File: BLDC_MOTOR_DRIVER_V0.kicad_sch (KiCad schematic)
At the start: 47 parts, among them J1 Conn_01x05_Pin, J10 Conn_01x01_Socket, J2 Conn_01x01_Socket, J3 Conn_01x01_Socket, J4 Conn_01x01_Socket, J5 Conn_01x01_Socket, J6 Conn_01x01_Socket, J7 Conn_01x01_Socket, J8 Conn_01x01_Socket, J9 Conn_01x01_Socket, Q1 N-MOSFET, Q2 N-MOSFET, Q3 N-MOSFET, Q4 N-MOSFET, Q5 N-MOSFET, Q6 N-MOSFET, U1 3-phase Gate Driver, U2 Micro controller, U3 3.3V Regurator

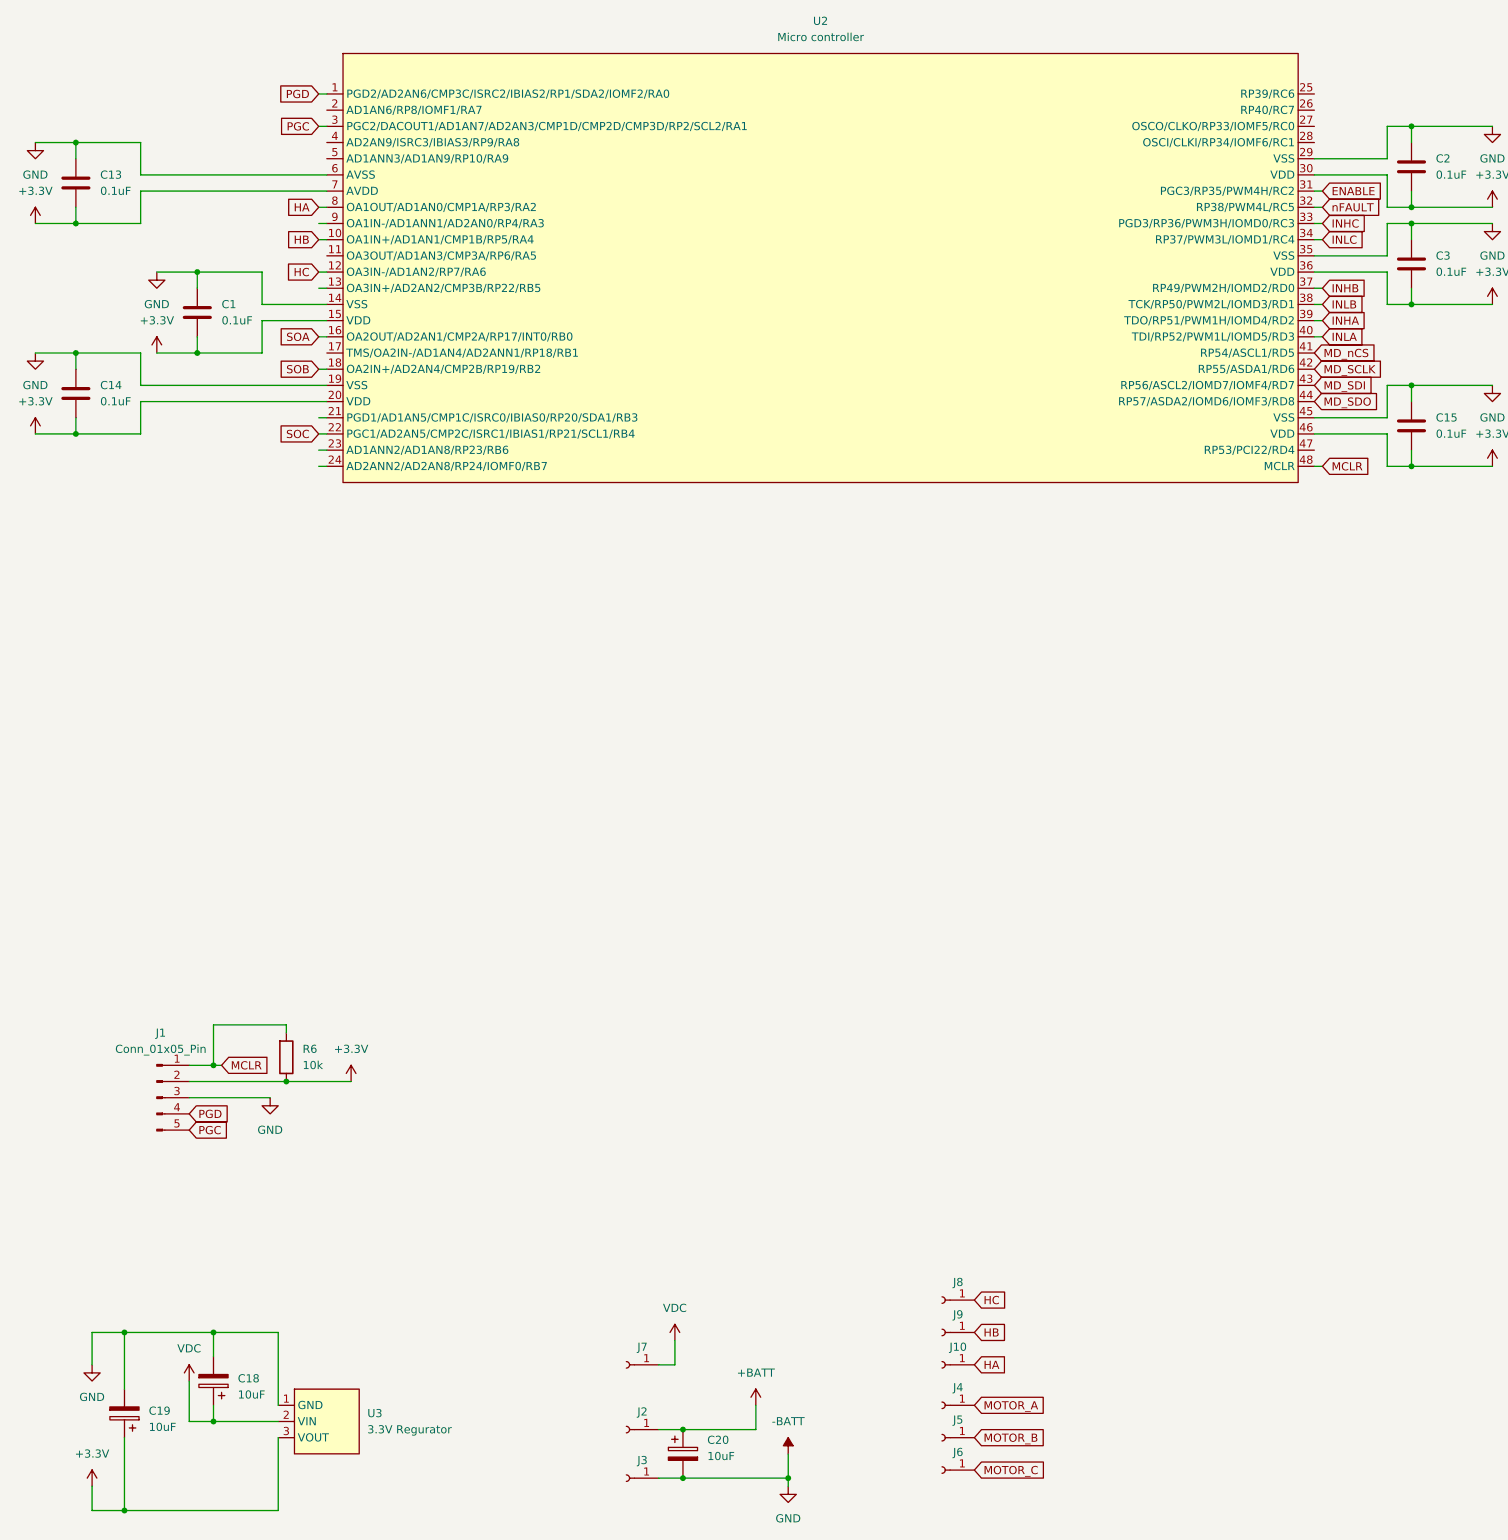
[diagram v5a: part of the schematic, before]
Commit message: up
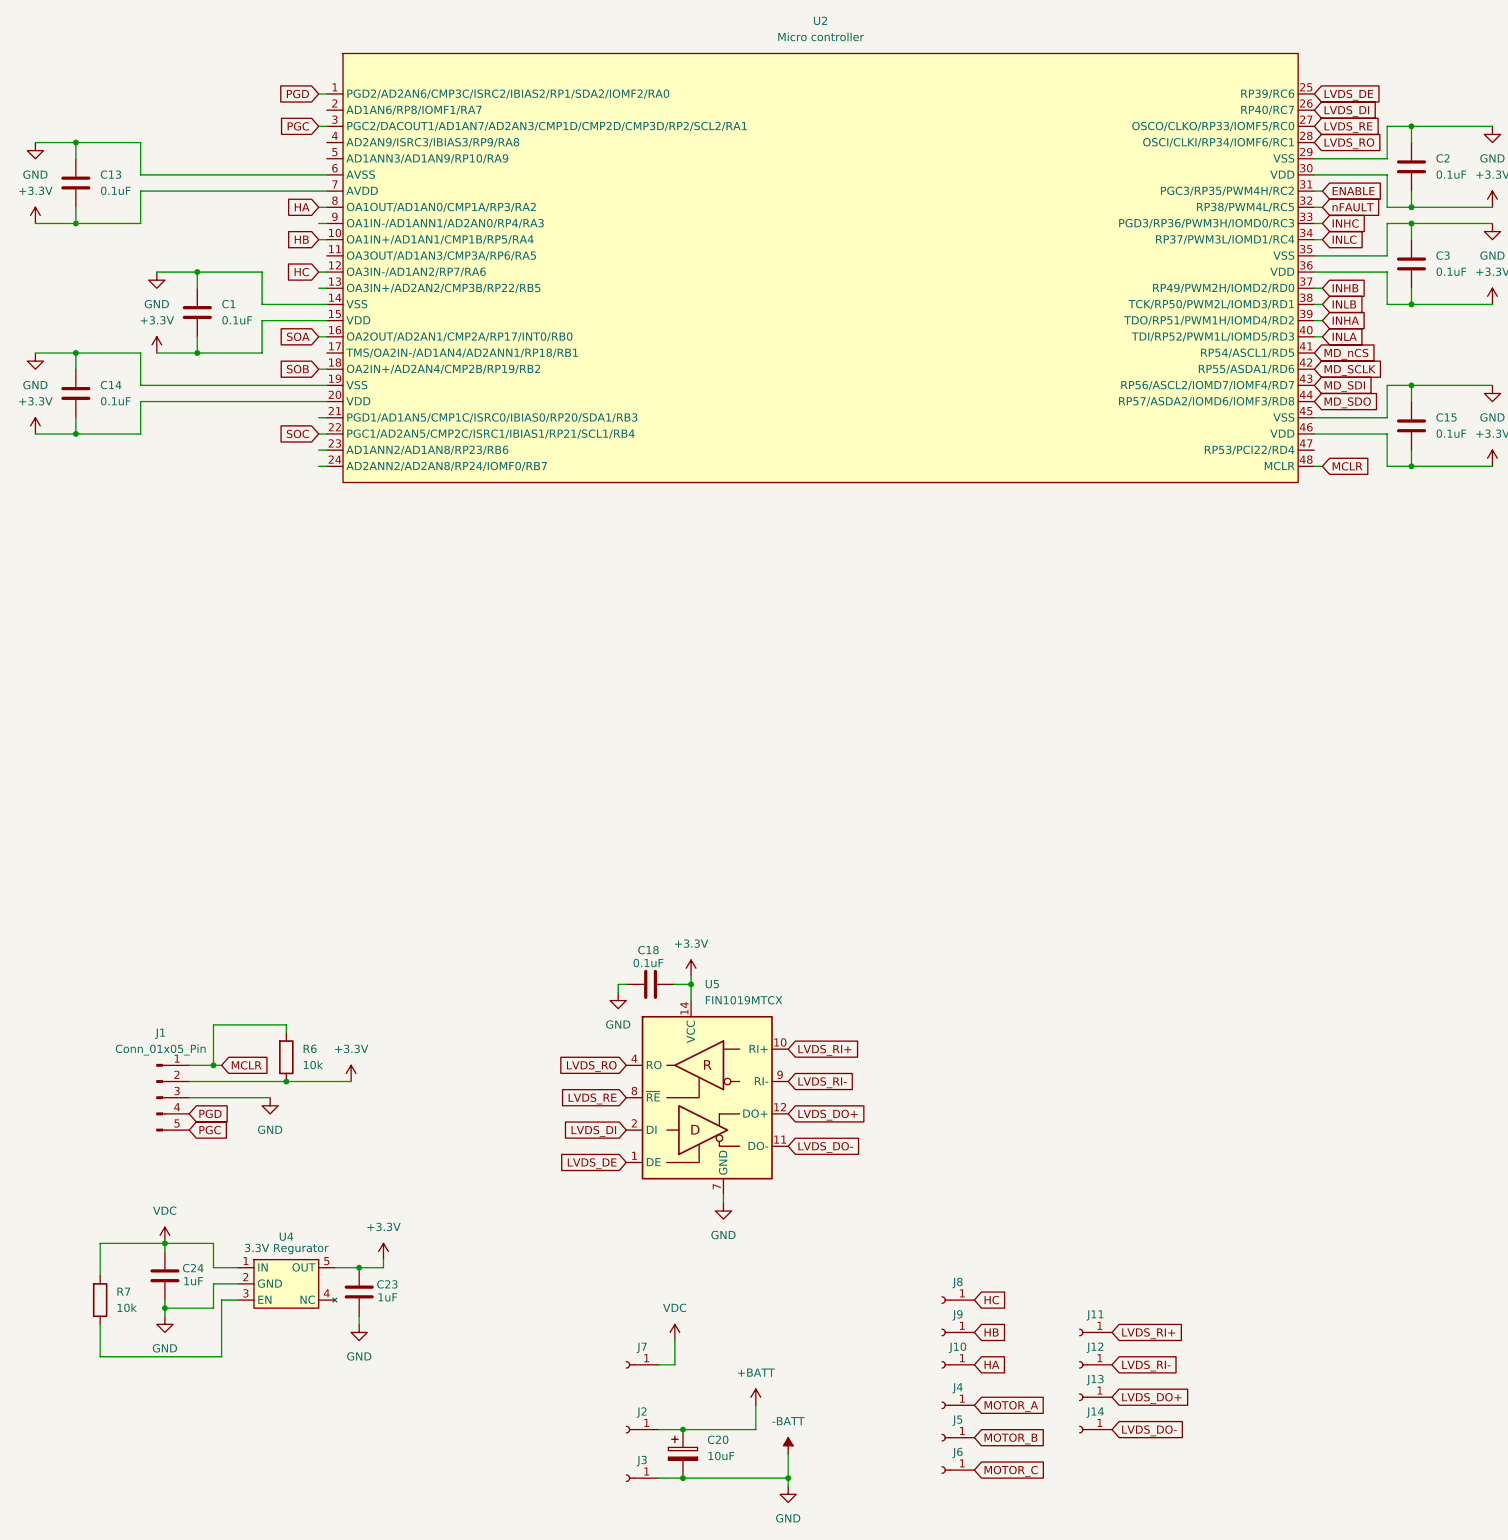
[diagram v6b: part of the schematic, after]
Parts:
- removed C18, C19: 10uF, Capacitor_SMD:C_Elec_5x5.4, symbol EMK1VM100D80D00R:EMK1VM100D80D00R
- removed U3: 3.3V Regurator, Package_TO_SOT_SMD:SOT-89-3, symbol SL7333-8:SL7333-8
- added C18: 0.1uF, Capacitor_SMD:C_0603_1608Metric, symbol GRM188F11H104ZA01:GRM188F11H104ZA01
- added C23, C24: 1uF, Capacitor_SMD:C_0805_2012Metric, symbol CL21B105KBFNNNE:CL21B105KBFNNNE
- added J11, J12, J13, J14: Conn_01x01_Socket, Connector_Wire:SolderWirePad_1x01_SMD_2x4mm, symbol Connector:Conn_01x01_Socket
- added R7: 10k, Resistor_SMD:R_0603_1608Metric, symbol NRC06F1002TRF:NRC06F1002TRF
- added U4: 3.3V Regurator, Package_TO_SOT_SMD:SOT-23-5, symbol TLV74033PDBVR:TLV74033PDBVR
- added U5: FIN1019MTCX, Package_SO:TSSOP-14_4.4x5mm_P0.65mm, symbol FIN1019MTCX:FIN1019MTCX
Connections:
- net +3.3V: now also C18.1, C23.1, U4.5 (OUT), U5.14 (VCC)
- net -BATT: now also C18.2, C23.2, C24.2, U4.2 (GND), U5.7 (GND)
- net VDC: now also C24.1, R7.1, U4.1 (IN)
- net LVDS_DE: now reaches U2.25 (RP39/RC6)
- net LVDS_DE: now also U5.1 (DE)
- net LVDS_DI: now reaches U2.26 (RP40/RC7)
- net LVDS_DI: now also U5.2 (DI)
- net LVDS_RE: now reaches U2.27 (OSCO/CLKO/RP33/IOMF5/RC0)
- net LVDS_RE: now also U5.8 (~{RE})
- net LVDS_RO: now reaches U2.28 (OSCI/CLKI/RP34/IOMF6/RC1)
- net LVDS_RO: now also U5.4 (RO)
- new net: R7.2, U4.3 (EN)
- new net LVDS_DO+: J13.1 (Pin_1), U5.12 (DO+)
- new net LVDS_DO-: J14.1 (Pin_1), U5.11 (DO-)
- new net LVDS_RI+: J11.1 (Pin_1), U5.10 (RI+)
- new net LVDS_RI-: J12.1 (Pin_1), U5.9 (RI-)
